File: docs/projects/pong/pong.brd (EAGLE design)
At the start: 66 x 50.5 mm, 19 parts, among them Q1 20MHz, X3 AUDIO, X4 VIDEO

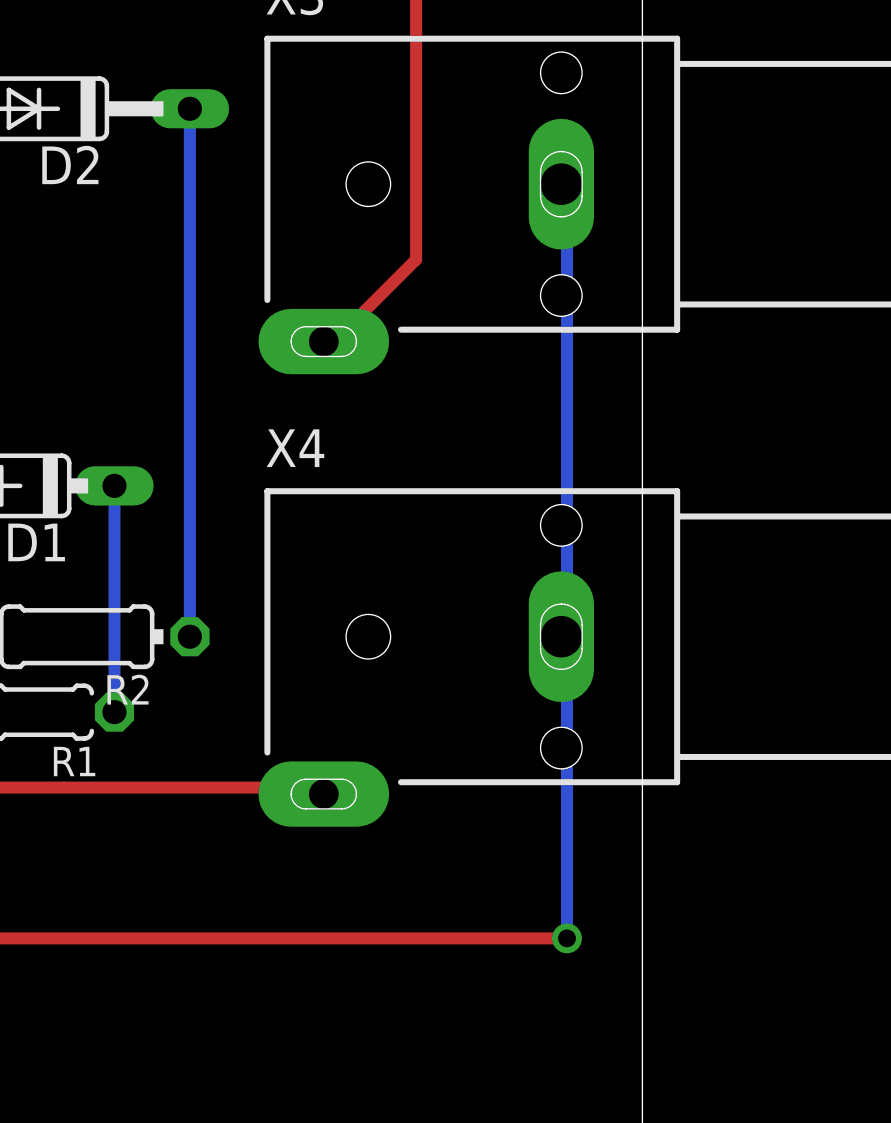
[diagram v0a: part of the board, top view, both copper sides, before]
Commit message: fix airwires
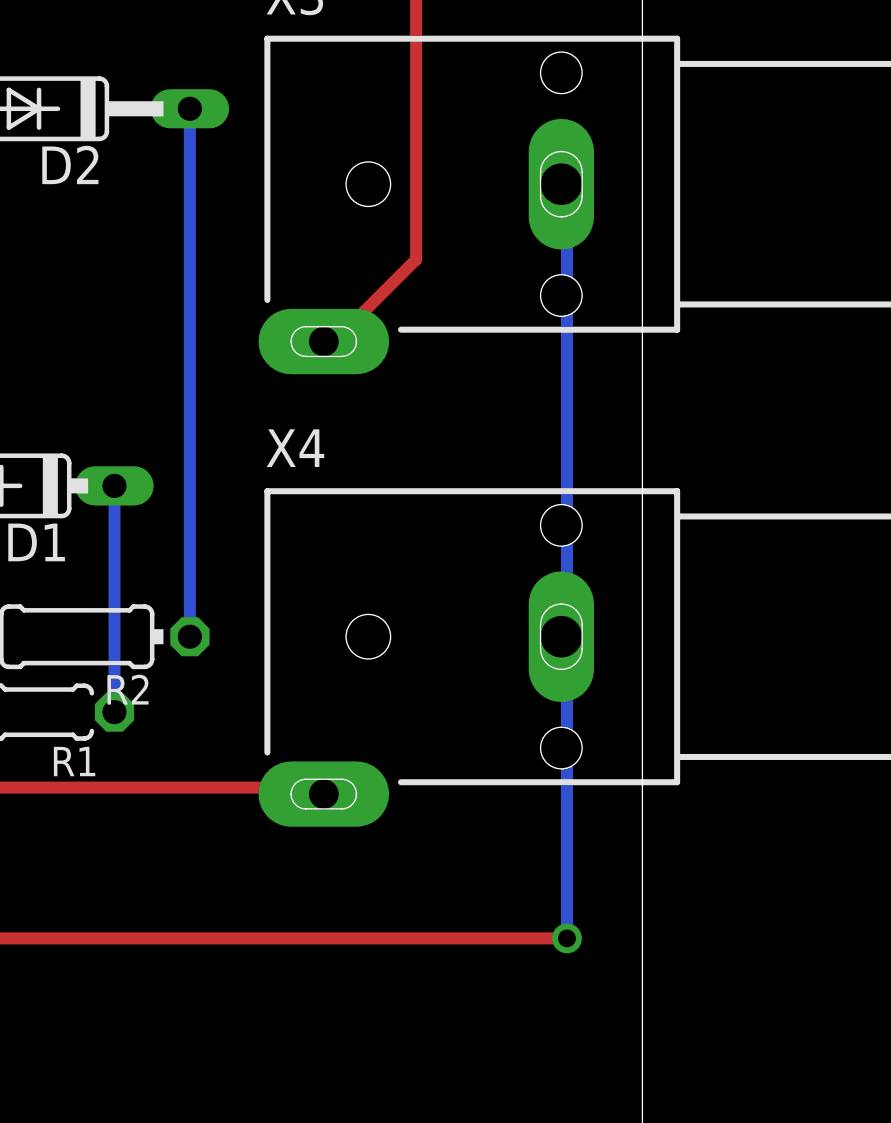
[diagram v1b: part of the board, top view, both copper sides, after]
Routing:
- net GND: track 153.7 -> 164.2 mm
- net N$15: track 41.7 -> 42.5 mm
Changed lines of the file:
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@@
 <setting verticaltext="up"/>
 </settings>
-<grid distance="0.1" unitdist="inch" unit="inch" style="lines" multiple="1" display="yes" altdistance="0.05" altunitdist="inch" altunit="inch"/>
+<grid distance="0.1" unitdist="inch" unit="inch" style="lines" multiple="1" display="no" altdistance="0.05" altunitdist="inch" altunit="inch"/>
 <layers>
 <layer number="1" name="Top" color="4" fill="1" visible="yes" active="yes"/>
@@
 <wire x1="60.96" y1="43.18" x2="60.96" y2="33.02" width="0.4064" layer="1"/>
 <wire x1="60.96" y1="33.02" x2="58.42" y2="30.48" width="0.4064" layer="1"/>
-<wire x1="57.85" y1="30.26" x2="58.42" y2="30.48" width="0" layer="19" extent="1-1"/>
+<wire x1="57.85" y1="30.26" x2="58.42" y2="30.26" width="0.4064" layer="1"/>
+<wire x1="58.42" y1="30.26" x2="58.42" y2="30.48" width="0.4064" layer="1"/>
 </signal>
 <signal name="N$11">
@@
 <wire x1="27.6606" y1="5.1054" x2="27.6606" y2="10.16" width="0.4064" layer="16"/>
 <wire x1="27.6606" y1="10.16" x2="27.94" y2="10.16" width="0.4064" layer="16"/>
-<wire x1="66.04" y1="35.56" x2="65.85" y2="35.56" width="0" layer="19" extent="16-16"/>
-<wire x1="65.85" y1="20.32" x2="66.04" y2="10.16" width="0" layer="19" extent="16-16"/>
+<wire x1="65.85" y1="20.32" x2="66.04" y2="20.32" width="0.4064" layer="16"/>
+<wire x1="66.04" y1="20.32" x2="66.04" y2="10.16" width="0.4064" layer="16"/>
+<wire x1="65.85" y1="35.56" x2="66.04" y2="35.56" width="0.4064" layer="16"/>
 </signal>
 <signal name="+5V">
